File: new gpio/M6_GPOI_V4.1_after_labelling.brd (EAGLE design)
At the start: 102.3 x 71.5 mm, 36 parts, among them IC4 LT1161, Q5 16MHz, Q8 16MHz, U3 MCP2515, U4 ATMEGA328P_PDIP, X2 MABC96R

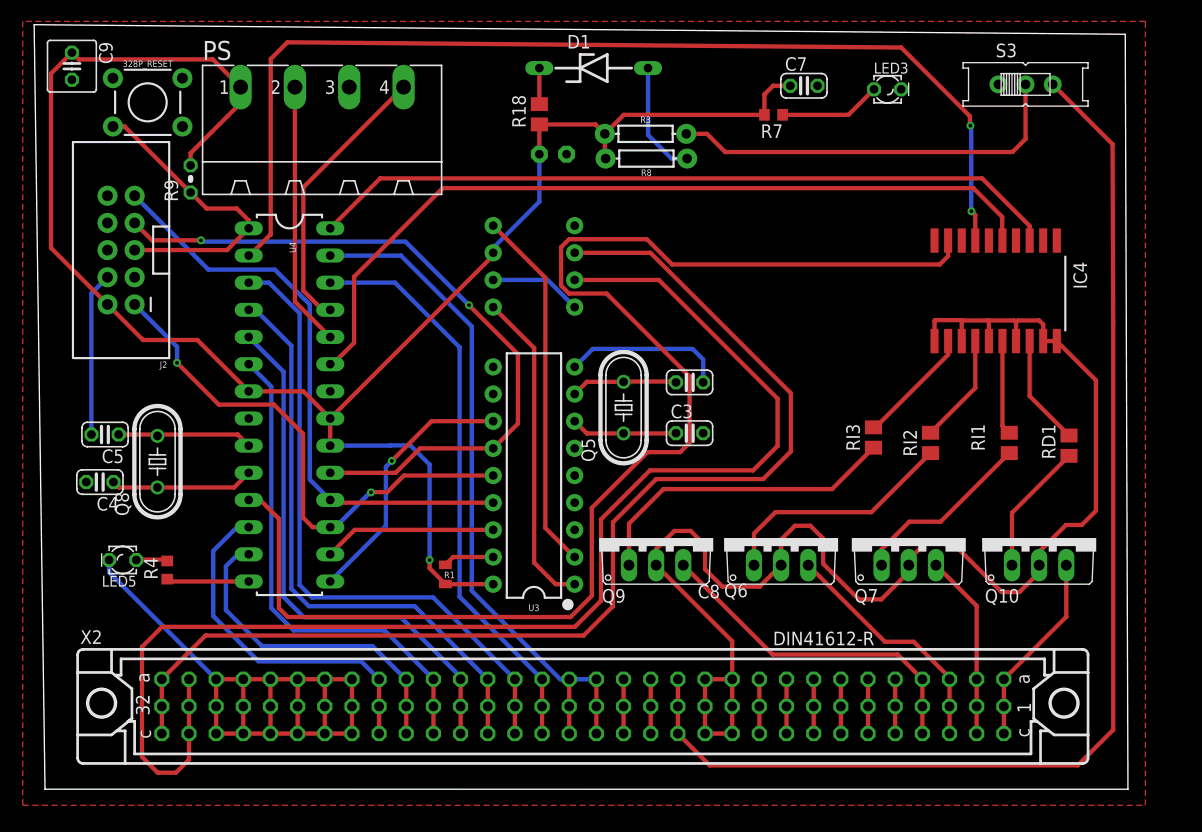
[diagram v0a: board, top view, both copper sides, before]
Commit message: gpio with nobi's changes
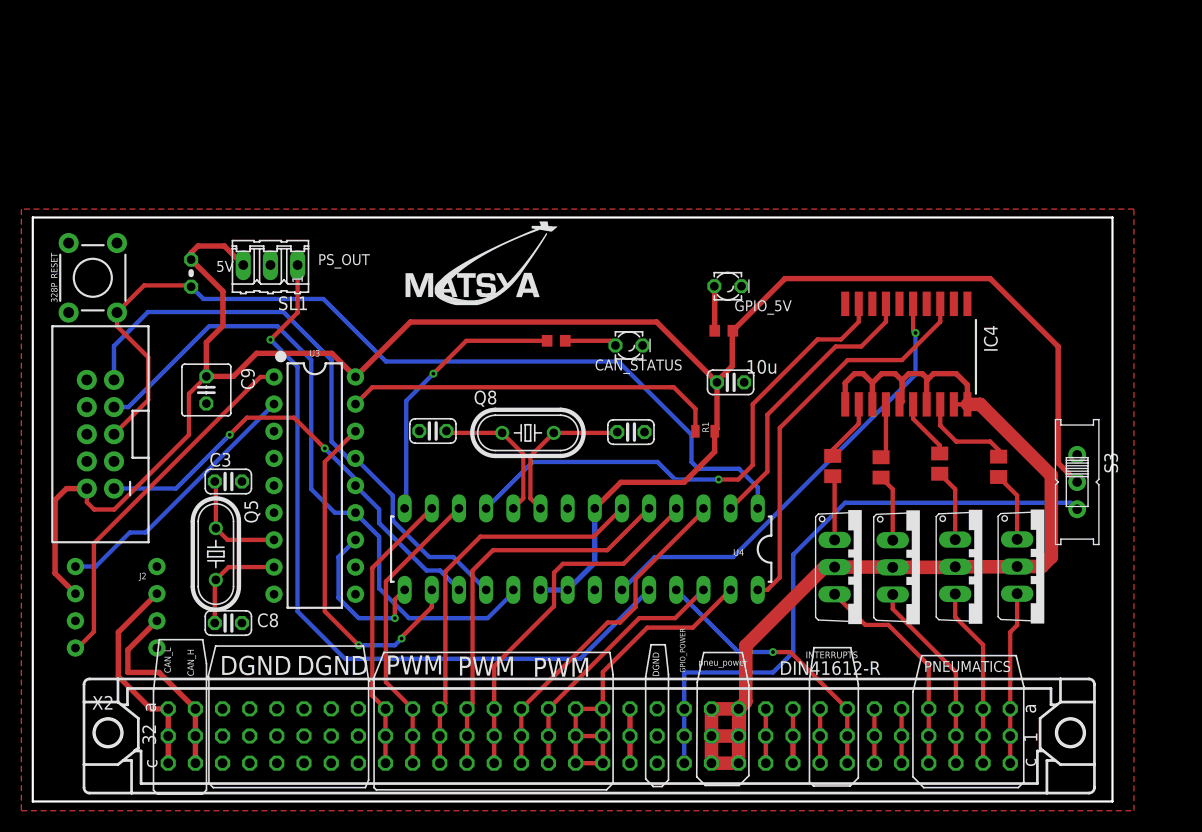
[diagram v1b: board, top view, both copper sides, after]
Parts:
- removed C1: (no value), capacitor-wima:C2.5-3
- removed D1: 5v, diode:ZDIO-10
- removed LED3, LED5: (no value), eagle-ltspice:LED_LD260
- removed PS: MSTBA4, con-phoenix-508:MSTBA4
- removed R18: (no value), rcl:M0805
- removed R3: 2.2k, SparkFun-Resistors:AXIAL-0.3
- removed R8: 0.732k, SparkFun-Resistors:AXIAL-0.3
- added CAN_STATUS, GPIO_5V: (no value), eagle-ltspice:LED_LD260
- added SL1: (no value), con-amp-quick:03P
- moved U$3 50.4 mm to (4.62, 15.6)
- moved C5 49.2 mm to (52.8, 32.0), turned to 0 degrees
- moved C8 48.6 mm to (15.1, 14.1)
- moved C3 43.4 mm to (15.1, 27.4)
- moved R4 42.2 mm to (45.8, 40.5), turned to 0 degrees
- moved Q5 40.5 mm to (13.9, 20.6), turned to 270 degrees
- moved S3 37.5 mm to (94.5, 27.3), turned to 270 degrees
- moved Q8 34.8 mm to (43.1, 31.9), turned to 0 degrees
- moved C9 32.8 mm to (13.1, 35.9)
- moved C4 31.5 mm to (34.2, 32.1)
- moved U4 30.4 mm to (48.1, 21.1), turned to 180 degrees
- moved C7 28.6 mm to (62.1, 36.7)
- moved R1 27.7 mm to (59.7, 32.1), turned to 180 degrees
- moved R7 20.7 mm to (61.4, 41.5), turned to 0 degrees
- moved U3 20.5 mm to (23.2, 27.0), turned to 270 degrees
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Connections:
- net CRY1 renamed CRY_N
- net CRY2 renamed CRY_P
- net N$10 renamed C_N
- net N$9 renamed C_P
- removed net BUFFER: PS.4, U4.25
- removed net GPIO_5V: C1.1, C7.1, C9.1, J2.2, PS.1, R1.1, R18.1, R3.P$1, R7.2, R8.P$2, R9.2, U$3.3, U3.18, U4.20, U4.21, U4.7
- removed net N$21: D1.C, R18.2
- net DGND: now also CAN_STATUS.K, GPIO_5V.K, SL1.2; no longer C1.2, D1.A, J2.4, J2.6, J2.8, LED3.K, LED5.K, PS.3, R8.P$1
- net GPIO_POWER: now also C7.1, C9.1, J2.2, R1.1, R7.2, R9.2, SL1.3, U$3.3, U3.18, U4.20, U4.21, U4.7; no longer R3.P$2
- net INT_1: now also U4.25
- net N$1: now also CAN_STATUS.A; no longer LED5.A
- net N$4: now also GPIO_5V.A; no longer LED3.A
- net PS_1: now also SL1.1; no longer PS.2
- net PWM1: now also U4.13; no longer U4.12
- net PWM2: now also U4.12; no longer U4.13
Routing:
- net GPIO_5V: track 171.8 -> 0.00 mm, vias 1 -> 0
- net GPIO_POWER: track 38.0 -> 191.5 mm
- net DGND: track 126.5 -> 0.00 mm
- net CAN1_P: track 123.0 -> 18.8 mm
- net CAN1_N: track 108.4 -> 20.2 mm
- net PNEU_4_IN: track 126.8 -> 48.4 mm, vias 0 -> 1
- net PNEU_3_IN: track 99.8 -> 26.5 mm, vias 2 -> 0
- net RESET: track 28.6 -> 86.2 mm
- net GPIO_POWER_IP: track 111.1 -> 57.4 mm
- net PS_1: track 24.7 -> 71.9 mm, vias 0 -> 1
- net PNEU_2_IN: track 76.7 -> 42.5 mm, vias 0 -> 1
- net PNEU_1_IN: track 70.6 -> 37.3 mm
- net N$8: track 4.77 -> 35.4 mm
- net PWM7: track 53.9 -> 24.2 mm
- net PWM8: track 65.9 -> 36.4 mm
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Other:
- board size 102.3 x 71.5 mm -> 101 x 54.6 mm
- board text added: "10u"
- board text added: "5V"
- board text added: "CAN_H"
- board text added: "CAN_L"
- board text added: "DGND"
- board text added: "GPIO_POWER"
- board text added: "INTERRUPTS"
- board text added: "PNEUMATICS"
- board text added: "PS_OUT"
- board text added: "PWM"
- board text added: "pneu_power"

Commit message: FINAL BY LK WITHOUT LABELLING
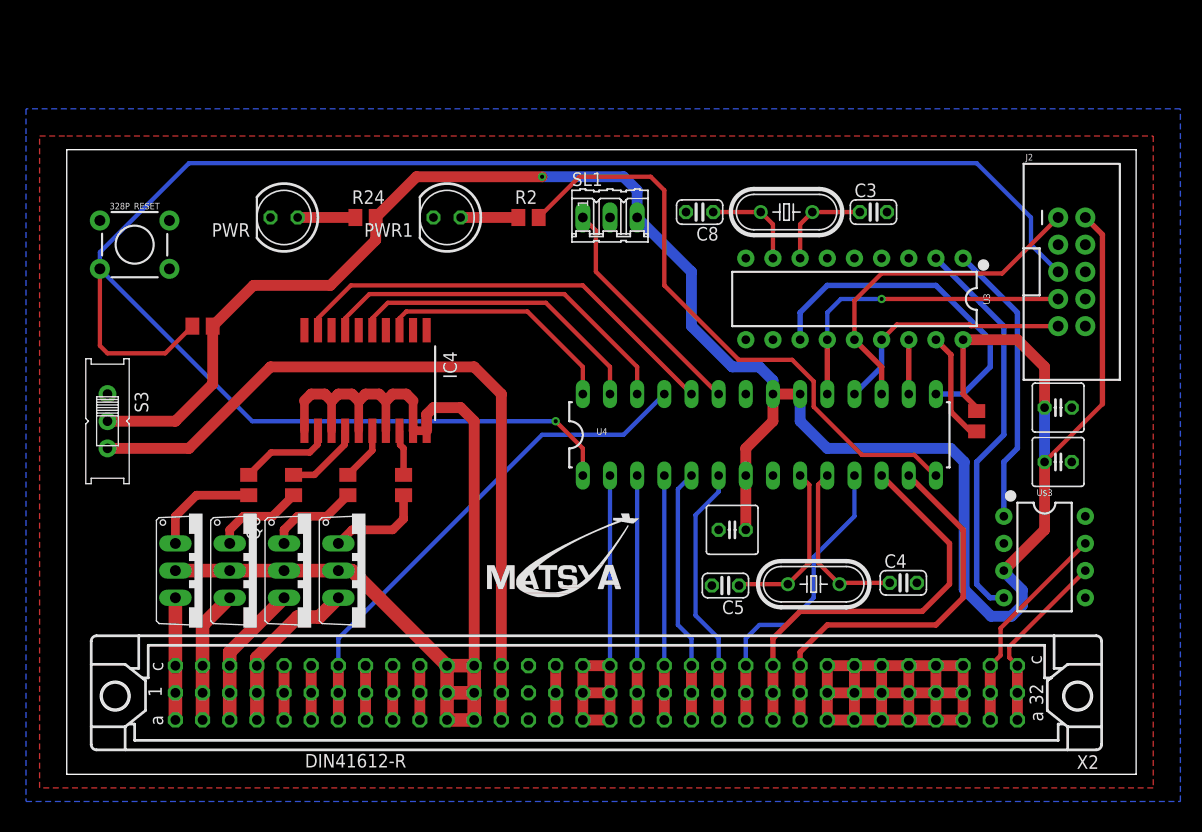
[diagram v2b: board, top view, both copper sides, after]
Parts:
- removed C7: 10u, resistor:C025-024X044
- removed CAN_STATUS, GPIO_5V: (no value), eagle-ltspice:LED_LD260
- removed R1: 10K, SparkFun-Resistors:0805
- removed R4, R7: 0.2k, adafruit:R0603
- removed R9: 10K, rcl:0204V
- added C1, C2: 10u, adafruit:C025-050X050
- added PWR, PWR1: (no value), led:LED5MM
- added R2, R24: 1k, rcl:M0805
- added RD2, RD3: 10K, rcl:M0805
- moved J2 92.1 mm to (94.0, 47.0), turned to 0 degrees
- moved S3 90.9 mm to (3.81, 33.0)
- moved U$3 86.9 mm to (91.4, 20.3), flipped to the top, turned to 270 degrees
- moved C9 79.7 mm to (92.7, 34.3), turned to 0 degrees
- moved Q10 78.7 mm to (12.7, 19.1)
- moved Q7 67.8 mm to (17.8, 19.1)
- moved C3 65.4 mm to (75.4, 52.6)
- moved Q5 62.2 mm to (67.3, 52.6), turned to 180 degrees
- moved C8 58.5 mm to (59.2, 52.6), turned to 180 degrees
- moved Q6 56.9 mm to (22.9, 19.1)
- moved RD1 55.7 mm to (31.5, 27.1)
- moved RI1 55.4 mm to (26.3, 27.1)
- moved RI2 55.0 mm to (21.2, 27.1)
- moved RI3 54.6 mm to (17.0, 27.1)
- moved U3 53.4 mm to (73.7, 44.5), turned to 180 degrees
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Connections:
- removed net N$4: GPIO_5V.A, R7.1
- new net N$31: PWR.A, R24.1
- net CAN_STAT_1: now also R2.2; no longer R4.1
- net DGND: now also C1.2, C2.2, PWR.K, PWR1.K; no longer C7.2, CAN_STATUS.K, GPIO_5V.K
- net GPIO_POWER: now also C1.1, C2.1, R24.2, RD2.2, RD3.1; no longer C7.1, R1.1, R7.2, R9.2
- net N$1: now also PWR1.A, R2.1; no longer CAN_STATUS.A, R4.2
- net N$8: now also RD2.1; no longer R1.2
- net PNEU_1_IN: now also IC4.9, U4.24; no longer IC4.3, U4.28
- net PNEU_1_OUT: now also RI3.1; no longer RD1.1
- net PNEU_2_IN: now also IC4.7, U4.26; no longer IC4.5, U4.23
- net PNEU_2_OUT: now also RI2.1; no longer RI1.1
- net PNEU_3_IN: now also IC4.5, U4.27; no longer IC4.7, U4.2
- net PNEU_3_OUT: now also RI1.1; no longer RI2.1
- net PNEU_4_IN: now also IC4.3, U4.28; no longer IC4.9, U4.11
- net PNEU_4_OUT: now also RD1.1; no longer RI3.1
- net PS_1: now also U4.23; no longer U4.24
- net PWM3: now also U4.11; no longer U4.6
- net PWM4: now also U4.6; no longer U4.5
- net PWM5: now also U4.5; no longer U4.4
- net PWM6: now also U4.4; no longer U4.3
- net PWM7: now also U4.3; no longer U4.26
- net PWM8: now also U4.2; no longer U4.27
- net RESET: now also RD3.2; no longer R9.1
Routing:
- net RESET: track 86.2 -> 172.1 mm, vias 0 -> 1
- net DGND: track 0.00 -> 68.6 mm
- net PS_1: track 71.9 -> 21.8 mm, vias 1 -> 0
- net CAN_SCK: track 62.9 -> 29.7 mm, vias 0 -> 1
- net CAN_MISO: track 55.9 -> 23.3 mm
- net CAN_STAT_1: track 25.6 -> 56.9 mm, vias 1 -> 0
- net CAN_SS: track 32.6 -> 5.08 mm, vias 2 -> 0
- net PNEU_4_IN: track 48.4 -> 23.2 mm, vias 1 -> 0
- net N$8: track 35.4 -> 10.5 mm
- net INT_1: track 25.7 -> 47.6 mm, vias 1 -> 0
- net GPIO_POWER: track 191.5 -> 210.5 mm, vias 0 -> 1
- net CAN_INT: track 15.2 -> 32.1 mm, vias 1 -> 0
- net GPIO_POWER_IP: track 57.4 -> 71.5 mm
- net PWM4: track 37.1 -> 24.6 mm
- net N$7: track 24.9 -> 37.2 mm
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- added copper zone on layer 16, net DGND
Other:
- board size 101 x 54.6 mm -> 100 x 58.4 mm
- board text removed: "10u"
- board text removed: "5V"
- board text removed: "CAN_H"
- board text removed: "CAN_L"
- board text removed: "DGND"
- board text removed: "GPIO_POWER"
- board text removed: "INTERRUPTS"
- board text removed: "PNEUMATICS"
- board text removed: "PS_OUT"
- board text removed: "PWM"
- board text removed: "pneu_power"
